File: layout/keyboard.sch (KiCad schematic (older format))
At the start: 113 parts, among them U1 ProMicro

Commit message: Updating with latest stuff
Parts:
- K_SPACE1, K_SPACE2: footprint MX_Only:MXOnly-2.25U-NoLED -> MX_Only:MXOnly-2.25U-ReversedStabilizers-NoLED
- U1: symbol keebio:ProMicro -> keyboard-rescue:ProMicro-keebio
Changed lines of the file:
@@
 F 0 "K_SPACE2" H 6500 5233 60  0000 C CNN
 F 1 "KEYSW" H 6500 4900 60  0001 C CNN
-F 2 "MX_Only:MXOnly-2.25U-NoLED" H 6500 5000 60  0001 C CNN
+F 2 "MX_Only:MXOnly-2.25U-ReversedStabilizers-NoLED" H 6500 5000 60  0001 C CNN
 F 3 "" H 6500 5000 60  0000 C CNN
 	1    6500 5000
@@
 F 0 "K_SPACE1" H 8500 5233 60  0000 C CNN
 F 1 "KEYSW" H 8500 4900 60  0001 C CNN
-F 2 "MX_Only:MXOnly-2.25U-NoLED" H 8500 5000 60  0001 C CNN
+F 2 "MX_Only:MXOnly-2.25U-ReversedStabilizers-NoLED" H 8500 5000 60  0001 C CNN
 F 3 "" H 8500 5000 60  0000 C CNN
 	1    8500 5000
@@
 	900  5400 2150 5400
 $Comp
-L keebio:ProMicro U1
+L keyboard-rescue:ProMicro-keebio U1
 U 1 1 602F1431
 P 7650 8050
@@
 col5
 $Comp
-L power:GND #PWR?
+L power:GND #PWR0101
 U 1 1 60410D36
 P 8850 7600
-F 0 "#PWR?" H 8850 7350 50  0001 C CNN
+F 0 "#PWR0101" H 8850 7350 50  0001 C CNN
 F 1 "GND" H 8855 7427 50  0000 C CNN
 F 2 "" H 8850 7600 50  0001 C CNN
@@
 	8350 7600 8850 7600
 $Comp
-L power:GND #PWR?
+L power:GND #PWR0102
 U 1 1 6049377B
 P 6600 7700
-F 0 "#PWR?" H 6600 7450 50  0001 C CNN
+F 0 "#PWR0102" H 6600 7450 50  0001 C CNN
 F 1 "GND" H 6605 7527 50  0000 C CNN
 F 2 "" H 6600 7700 50  0001 C CNN

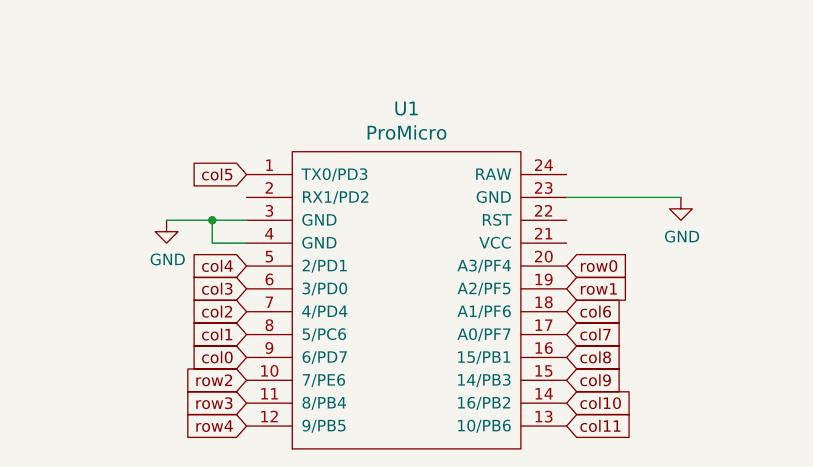
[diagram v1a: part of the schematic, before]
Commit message: add 60% version
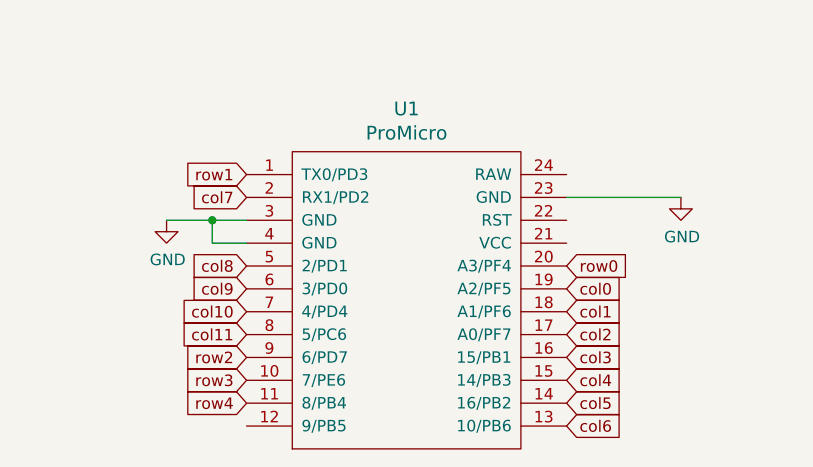
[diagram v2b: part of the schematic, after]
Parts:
- D_0, D_1, D_2, D_3, D_4, D_5, D_6, D_7, D_8, D_9, D_A1, D_ALT1, D_B1, D_BKSP1, D_BSLSH1, D_C1, D_CBRAC1, D_COMMA1, D_CTRL1, D_D1, D_DOT1, D_E1, D_EQUAL1, D_ESC1, D_F1, D_G1, D_H1, D_I1, D_J1, D_K1, D_L1, D_M1, D_MINUS1, D_N1, D_O1, D_OBRAC1, D_P1, D_Q1, D_QUOTE1, D_R1, D_S1, D_SEMIC1, D_SHIFT1, D_SLASH1, D_SPACE1, D_SPACE2, D_SUPER1, D_T1, D_TAB1, D_U1, D_V1, D_W1, D_X1, D_Y1, D_Z1, D_`1: footprint keyboard_parts:D_SOD123_axial -> Diode_SMD:D_SOD-123
- K_0, K_1, K_2, K_3, K_4, K_5, K_6, K_7, K_8, K_9, K_A1, K_B1, K_C1, K_CBRAC1, K_COMMA1, K_D1, K_DOT1, K_E1, K_EQUAL1, K_ESC1, K_F1, K_G1, K_H1, K_I1, K_J1, K_K1, K_L1, K_M1, K_MINUS1, K_N1, K_O1, K_OBRAC1, K_P1, K_Q1, K_QUOTE1, K_R1, K_S1, K_SEMIC1, K_SLASH1, K_T1, K_U1, K_V1, K_W1, K_X1, K_Y1, K_Z1, K_`1: footprint MX_Only:MXOnly-1U-NoLED -> MX_Only:MXOnly-1U-Hotswap
- K_ALT1, K_SUPER1: footprint MX_Only:MXOnly-1.25U-NoLED -> MX_Only:MXOnly-1.25U-Hotswap
- K_BKSP1: footprint MX_Only:MXOnly-2U-NoLED -> MX_Only:MXOnly-2U-Hotswap
- K_BSLSH1, K_TAB1: footprint MX_Only:MXOnly-1.5U-NoLED -> MX_Only:MXOnly-1.5U-Hotswap
- K_CTRL1: footprint MX_Only:MXOnly-1.75U-NoLED -> MX_Only:MXOnly-1U-Hotswap
- K_SHIFT1: footprint MX_Only:MXOnly-2.25U-NoLED -> MX_Only:MXOnly-2.25U-Hotswap
- K_SPACE1, K_SPACE2: footprint MX_Only:MXOnly-2.25U-ReversedStabilizers-NoLED -> MX_Only:MXOnly-2.25U-Hotswap-ReversedStabilizers
- U1: footprint Keebio-Parts:ArduinoProMicro -> Keebio-Parts:ArduinoProMicro-ZigZag
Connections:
- net col0: now also U1.19 (A2/PF5); no longer U1.9 (6/PD7)
- net col1: now also U1.18 (A1/PF6); no longer U1.8 (5/PC6)
- net col10: now also U1.7 (4/PD4); no longer U1.14 (16/PB2)
- net col11: now also U1.8 (5/PC6); no longer U1.13 (10/PB6)
- net col2: now also U1.17 (A0/PF7); no longer U1.7 (4/PD4)
- net col3: now also U1.16 (15/PB1); no longer U1.6 (3/PD0)
- net col4: now also U1.15 (14/PB3); no longer U1.5 (2/PD1)
- net col5: now also U1.14 (16/PB2); no longer U1.1 (TX0/PD3)
- net col6: now also U1.13 (10/PB6); no longer U1.18 (A1/PF6)
- net col7: now also U1.2 (RX1/PD2); no longer U1.17 (A0/PF7)
- net col8: now also U1.5 (2/PD1); no longer U1.16 (15/PB1)
- net col9: now also U1.6 (3/PD0); no longer U1.15 (14/PB3)
- net row1: now also U1.1 (TX0/PD3); no longer U1.19 (A2/PF5)
- net row2: now also U1.9 (6/PD7); no longer U1.10 (7/PE6)
- net row3: now also U1.10 (7/PE6); no longer U1.11 (8/PB4)
- net row4: now also U1.11 (8/PB4); no longer U1.12 (9/PB5)
